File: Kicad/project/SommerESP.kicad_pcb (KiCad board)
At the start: 2 copper layers, 41.7 x 48.6 mm, 37 parts, among them J1 Serial programmer, J2 BRIDGE CONEX, J3 SOMMER CONEX BOARD, J4 SOMMER CONEX KEYPAD, J5 BRIDGE POWER, J6 SOMMER OUTPUT OC, Q1 STN3NF06, Q2 2N7002DW, U4 LM2596SX-3.3/NOPB, U5 ESP32-C3-WROOM-02

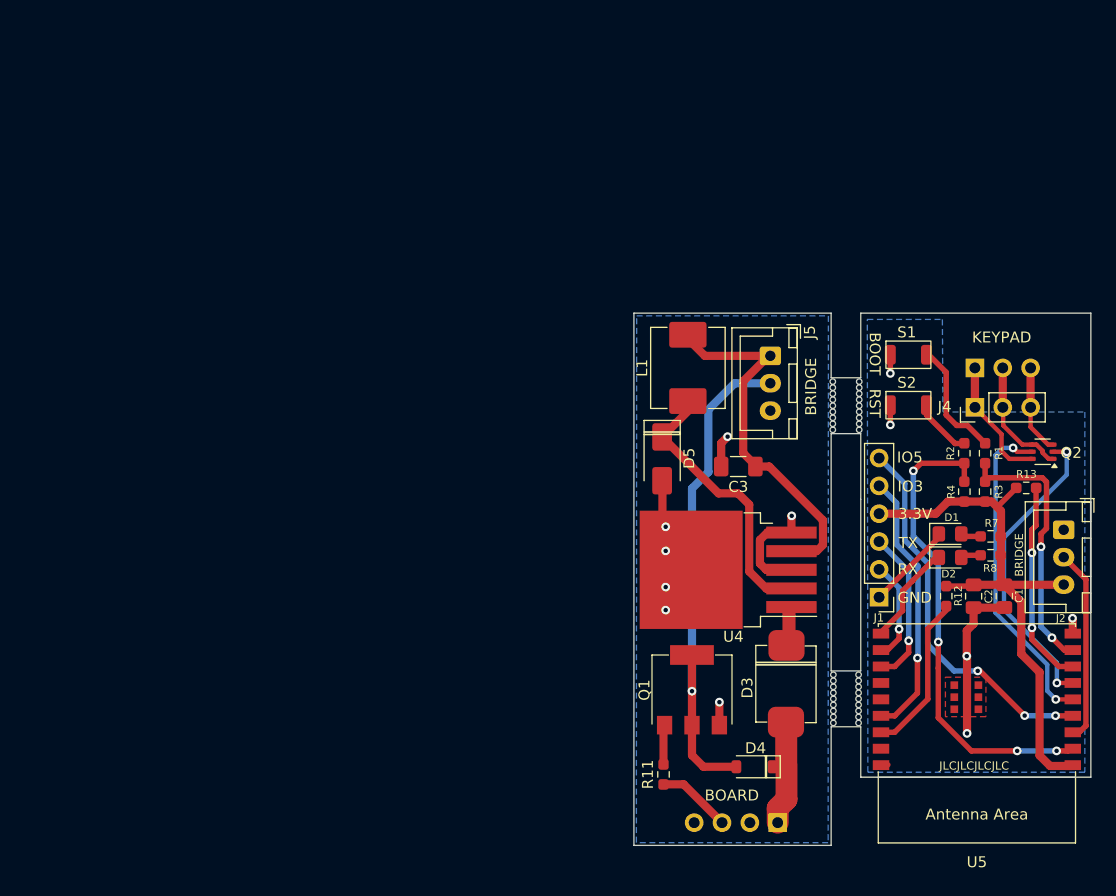
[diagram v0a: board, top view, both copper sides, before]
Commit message: Version 3.0 of SommerESP
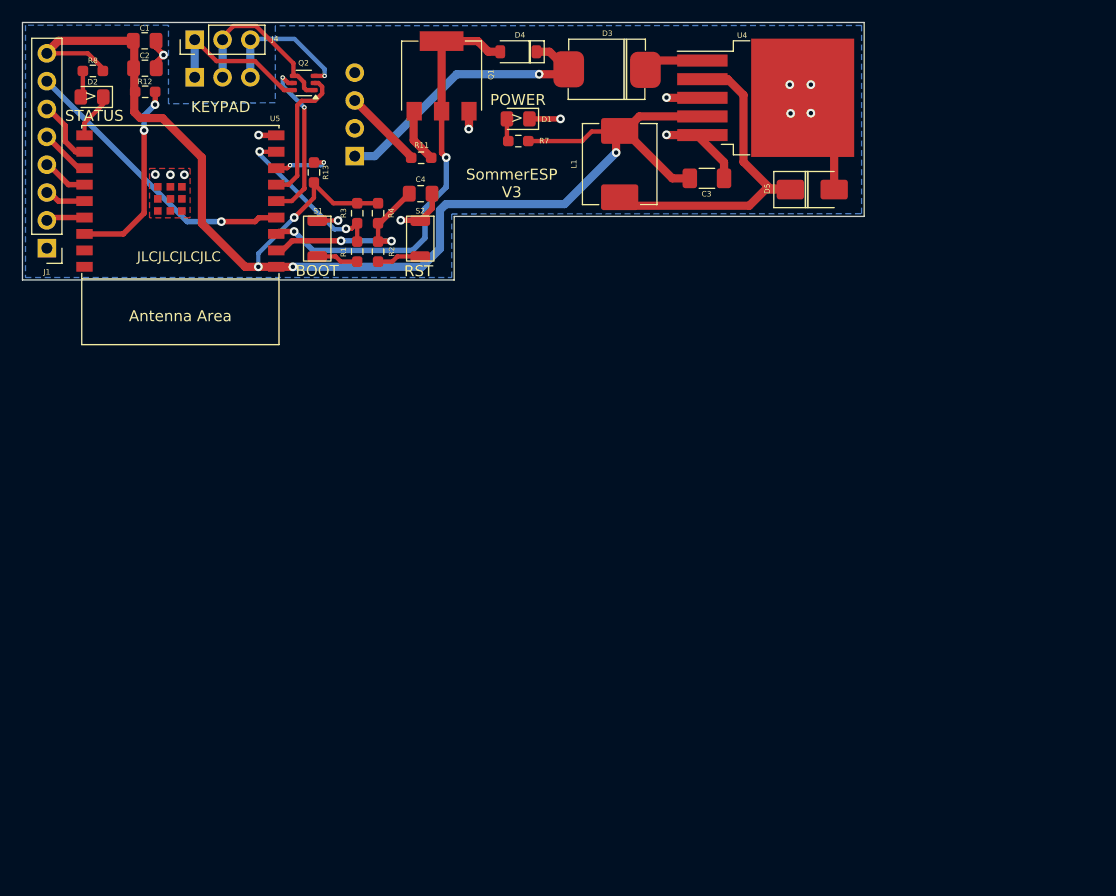
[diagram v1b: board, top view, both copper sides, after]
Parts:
- removed the G*** at (96.0, 83.3)
- removed H1, H2, H3, H4: MountingHole, CustomLibrary:Panelizing_1_1
- removed J2: BRIDGE CONEX, Connector_JST:JST_XH_B3B-XH-A_1x03_P2.50mm_Vertical
- removed J5: BRIDGE POWER, Connector_JST:JST_XH_B3B-XH-A_1x03_P2.50mm_Vertical
- added C4: 0805 22uf, Capacitor_SMD:C_0805_2012Metric_Pad1.18x1.45mm_HandSolder, F.Cu at (69.7, 40.1)
- D1: value LED GREEN -> LED Green
- D2: value LED BLUE -> LED Blue
- J1: footprint Connector_PinHeader_2.54mm:PinHeader_1x06_P2.54mm_Vertical -> Connector_PinHeader_2.54mm:PinHeader_1x08_P2.54mm_Vertical
- U4: value LM2596SX-3.3/NOPB -> LM2596SX-3.3/NOPB
- moved C1 93.4 mm to (44.5, 26.1), turned to 0 degrees
- moved R8 93.1 mm to (39.8, 28.9)
- moved C2 89.7 mm to (44.6, 28.6), turned to 0 degrees
- moved D2 88.9 mm to (39.8, 31.3), turned to 180 degrees
- moved R12 86.4 mm to (44.6, 30.8), turned to 180 degrees
- moved U5 85.7 mm to (47.8, 40.9)
- moved J1 82.4 mm to (35.6, 45.1)
- moved J4 78.7 mm to (49.1, 26.1)
- moved J3 76.0 mm to (49.1, 29.5)
- moved Q2 75.4 mm to (59.1, 30.0)
- moved J6 72.0 mm to (63.7, 36.7), turned to 0 degrees
- moved G*** 71.9 mm to (73.5, 37.5), turned to 180 degrees
- moved R13 71.1 mm to (60.0, 38.2), turned to -90 degrees
- moved D4 68.7 mm to (78.7, 27.1)
- moved R3 62.7 mm to (64.0, 41.9), turned to 90 degrees
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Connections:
- C1 pad 1: +3.3VA -> +3.3V
- C1 pad 2: GND2 -> GND
- C2 pad 1: +3.3VA -> +3.3V
- C2 pad 2: GND2 -> GND
- D1 pad 1: GND2 -> GND
- J1 pad 1: GND2 -> GND
- J1 pad 2: RX -> IO3
- J1 pad 3: TX -> IO19
- J1 pad 4: +3.3VA -> IO18
- J1 pad 5: IO3 -> TX
- J1 pad 6: IO5 -> RX
- R12 pad 2: +3.3VA -> +3.3V
- R13 pad 2: +3.3VA -> +3.3V
- R3 pad 2: +3.3VA -> +3.3V
- R4 pad 2: +3.3VA -> +3.3V
- R7 pad 1: +3.3VA -> +3.3V
- R8 pad 1: +3.3VA -> +3.3V
- S1 pad 2: GND2 -> GND
- S2 pad 2: GND2 -> GND
- U5 pad 1: +3.3VA -> +3.3V
- U5 pad 13: unconnected-(U5-GPIO18/USB_D--Pad13) -> IO18
- U5 pad 14: unconnected-(U5-GPIO19/USB_D+-Pad14) -> IO19
- U5 pad 19: GND2 -> GND
- U5 pad 3: ANALOGSIG2 -> AnalogSIG
- U5 pad 9: GND2 -> GND
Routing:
- net +3.3V: track 32.9 -> 120.3 mm, vias 0 -> 4
- net +3.3VA: track 51.8 -> 0.00 mm
- net GND2: track 27.1 -> 0.00 mm, vias 5 -> 0
- net EN: track 43.1 -> 17.5 mm, vias 4 -> 2
- net IO3: track 24.6 -> 3.58 mm, vias 1 -> 0
- net ANALOGSIG2: track 17.9 -> 0.00 mm
- net IO7: track 28.2 -> 12.9 mm, vias 2 -> 0
- net +24V: track 9.26 -> 24.2 mm, vias 0 -> 1
- net IO6: track 30.1 -> 15.3 mm
- net IO8: track 18.4 -> 5.27 mm
- net GND: track 19.4 -> 30.4 mm, vias 7 -> 15
- net TX: track 14.5 -> 4.35 mm, vias 1 -> 0
- net IO9: track 24.6 -> 15.1 mm
- net IO5: track 34.8 -> 26.1 mm, vias 3 -> 1
- net AnalogSIG: track 46.3 -> 37.6 mm, vias 1 -> 2
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- added copper zone on F.Cu, net GND
- removed copper zone on B.Cu, net GND2
- removed copper zone on F.Cu, net GND2
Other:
- board size 41.7 x 48.6 mm -> 76.8 x 23.5 mm
- board text added: ">"
- board text added: "IO18"
- board text added: "IO19"
- board text added: "POWER"
- board text added: "STATUS"
- board text added: "SommerESP V3"
- board text added: "SommerESP v3.0"
- board text removed: "BOARD"
- board text removed: "BRIDGE"
- board text removed: "IO5 IO3 3.3V TX RX GND"
- board text removed: "SommerESP v2.0 Control board"
- board text removed: "SommerESP v2.0 Power board"
